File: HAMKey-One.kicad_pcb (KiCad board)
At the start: 2 copper layers, 61 x 60.2 mm, 53 parts, among them J1 Conn_01x04, Q1 DTC143Z, SW1 SW_Main, SW3 SW_PWR, U1 nRF52832-QFxx

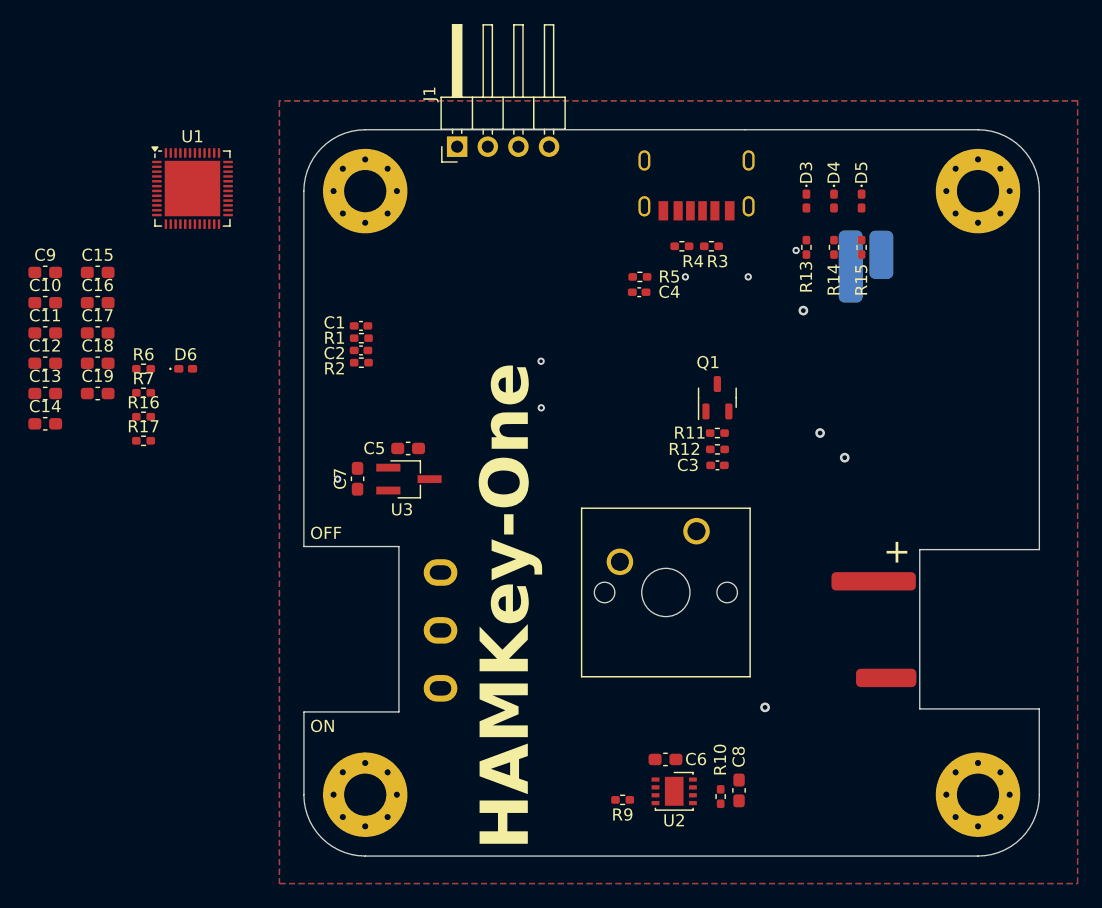
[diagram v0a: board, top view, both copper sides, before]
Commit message: near finish layout
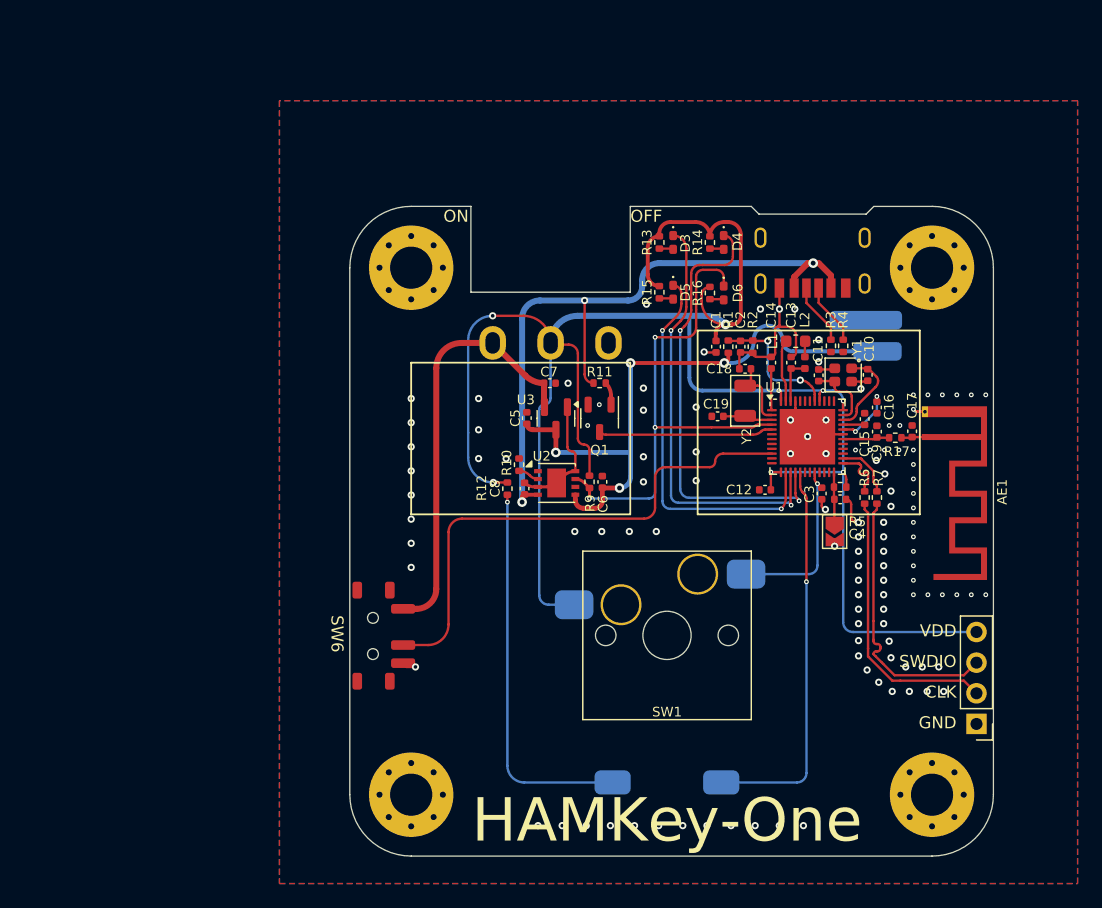
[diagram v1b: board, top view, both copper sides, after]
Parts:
- added AE1: Antenna_Shield, RF_Antenna:Texas_SWRA117D_2.4GHz_Right, F.Cu at (168.1, 95.7)
- added L1: 10uH, Inductor_SMD:L_0603_1608Metric, F.Cu at (157.4, 87.8)
- added L2: 15nH, Inductor_SMD:L_0402_1005Metric, F.Cu at (158.1, 89.5)
- added SW2: SW_Reset, Jumper:SolderJumper-2_P1.3mm_Open_TrianglePad1.0x1.5mm, F.Cu at (160.6, 103.5)
- added SW6: SW_SOUND, xianii:SK-3296S-01-L1, F.Cu at (122.3, 112.2)
- added Y1: Xtal_32M, PCM_Crystal_AKL:Crystal_SMD_2016-4Pin_2.0x1.6mm, F.Cu at (161.3, 90.6)
- added Y2: 32.768kHz, PCM_Crystal_AKL:Crystal_SMD_3215-2Pin_3.2x1.5mm, F.Cu at (153.2, 92.7)
- BATT1: footprint nigh_Library:BATT2030 -> xianii:BATT-501240
- BZ1: footprint nigh_Library:buzzer_SMD -> xianii:BUZZ-9032; moved to B.Cu
- C1, C2, C3, C4: footprint Capacitor_SMD:C_0402_1005Metric_Pad0.74x0.62mm_HandSolder -> Capacitor_SMD:C_0402_1005Metric
- C10, C11, C12, C13, C14, C15, C16, C17, C18, C19, C5, C6, C7, C8, C9: footprint Capacitor_SMD:C_0603_1608Metric_Pad1.08x0.95mm_HandSolder -> Capacitor_SMD:C_0402_1005Metric
- J1: footprint Connector_PinHeader_2.54mm:PinHeader_1x04_P2.54mm_Horizontal -> Connector_PinHeader_2.54mm:PinHeader_1x04_P2.54mm_Vertical
- R1, R10, R11, R12, R13, R14, R15, R16, R17, R2, R3, R4, R5, R6, R7, R9: footprint Resistor_SMD:R_0402_1005Metric_Pad0.72x0.64mm_HandSolder -> Resistor_SMD:R_0402_1005Metric
- SW1: footprint Button_Switch_Keyboard:SW_Cherry_MX_1.00u_PCB -> xianii:KEY-1511
- U2: value ~ -> SLM6400
- U3: footprint Package_TO_SOT_SMD:TSOT-23_HandSoldering -> Package_TO_SOT_SMD:SOT-23
- moved C9 70.2 mm to (164.1, 95.2), turned to 90 degrees
- moved C10 68.4 mm to (163.3, 90.6), turned to 90 degrees
- moved C17 68.0 mm to (167.0, 95.2), turned to 90 degrees
- moved C16 65.2 mm to (164.1, 93.2), turned to 90 degrees
- moved C15 64.7 mm to (163.1, 94.2), turned to -90 degrees
- moved J1 64.4 mm to (172.3, 119.5), turned to 180 degrees
- moved C11 64.2 mm to (159.3, 90.6), turned to -90 degrees
- moved R17 62.3 mm to (165.6, 95.8), turned to 180 degrees
- moved C13 61.9 mm to (157.0, 89.5), turned to 90 degrees
- moved R7 61.4 mm to (164.1, 100.7), turned to -90 degrees
- moved R6 60.7 mm to (163.1, 100.7), turned to -90 degrees
- moved C12 60.6 mm to (154.8, 100.1), turned to 180 degrees
- moved C14 60.4 mm to (155.3, 89.5), turned to -90 degrees
- moved U1 55.0 mm to (158.3, 95.7)
- moved C18 53.7 mm to (153.2, 90.0), turned to 180 degrees
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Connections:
- net /SWDCLK renamed /SWD+
- net /SWDIO renamed /SWD-
- net Net-(J1-Pin_2) renamed /SWDP
- net Net-(J1-Pin_3) renamed /SWDN
- C3 pad 2: /BTN -> /BTN0
- C7 pad 1: +3.3V -> LDO3v3
- C8 pad 1: +5V -> GND
- C8 pad 2: GND -> +5V
- D6 pad 1: /LED_GREEN -> /CHARGING
- R10 pad 1: Net-(U2-ISET) -> GND
- R10 pad 2: GND -> Net-(U2-PROG)
- SW1 pad 1: /BTN -> /BTN0
- SW3 pad 1: +3.3V -> LDO3v3
- SW3 pad 2: /ON/OFF -> +3.3V
- U1 pad 10: unconnected-(U1-P0.08-Pad10) -> /SW_SOUND
- U1 pad 17: /LED_GREEN -> /BUZZER
- U1 pad 19: unconnected-(U1-P0.16-Pad19) -> /BTN2
- U1 pad 20: unconnected-(U1-P0.17-Pad20) -> /BTN0
- U1 pad 8: /BTN -> unconnected-(U1-P0.06-Pad8)
- U1 pad 9: /BUZZER -> unconnected-(U1-P0.07-Pad9)
- U2 pad 1: /BAT+ -> unconnected-(U2-NTC-Pad1)
- U2 pad 2: unconnected-(U2-FULL-Pad2) -> Net-(U2-PROG)
- U2 pad 3: /CHARGING -> GND
- U2 pad 4: GND -> +5V
- U2 pad 5: GND -> /BAT+
- U2 pad 6: Net-(U2-ISET) -> unconnected-(U2-~{STDBY}-Pad6)
- U2 pad 7: unconnected-(U2-NC-Pad7) -> /CHARGING
- U2 pad 8: +5V -> GND
- U2 pad 9: (no net) -> GND
- U3 pad 2: +3.3V -> LDO3v3
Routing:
- net +3.3V: track 0.00 -> 167.5 mm, vias 7 -> 8
- net +5V: track 0.00 -> 57.1 mm
- net /BAT+: track 0.00 -> 51.8 mm, vias 0 -> 4
- net /SW_SOUND: track 0.00 -> 43.8 mm
- net /CHARGING: track 0.00 -> 42.3 mm, vias 0 -> 3
- net GND: track 0.00 -> 40.6 mm, vias 0 -> 116
- net /LED_BLUE: track 0.00 -> 37.4 mm, vias 0 -> 2
- net /LED_RED: track 0.00 -> 35.7 mm, vias 0 -> 2
- net LDO3v3: track 0.00 -> 35.2 mm
- net /BUZZER: track 0.00 -> 32.6 mm, vias 0 -> 1
- net /LED_WHITE: track 0.00 -> 32.1 mm, vias 0 -> 2
- net Net-(BZ1--): track 0.00 -> 31.9 mm, vias 0 -> 1
- net /SWDP: track 0.00 -> 23.0 mm
- net /SWDN: track 0.00 -> 23.0 mm
- net /BTN0: track 0.00 -> 15.5 mm, vias 0 -> 1
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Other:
- board size 61 x 60.2 mm -> 53.4 x 53.9 mm
- board text added: "Battery: 3.7V 130mAh Input: 5.0V 200mA"
- board text added: "CLK"
- board text added: "GND"
- board text added: "SWDIO"
- board text added: "VDD"
- board text added: "github.com/HAM-Key"
- board text removed: "Battery: 3.7V 300mAh Input: 5.0V 200mA"
- board text removed: "HelloWorks@GitHub"
- board text removed: "https://github.com/HAM-Key"
